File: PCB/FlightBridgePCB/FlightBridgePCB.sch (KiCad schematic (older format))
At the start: 11 parts, among them J1 Raspberry_Pi_2_3, J2 AVR-ISP-6, U1 ATmega128A-AU, Y1 Crystal

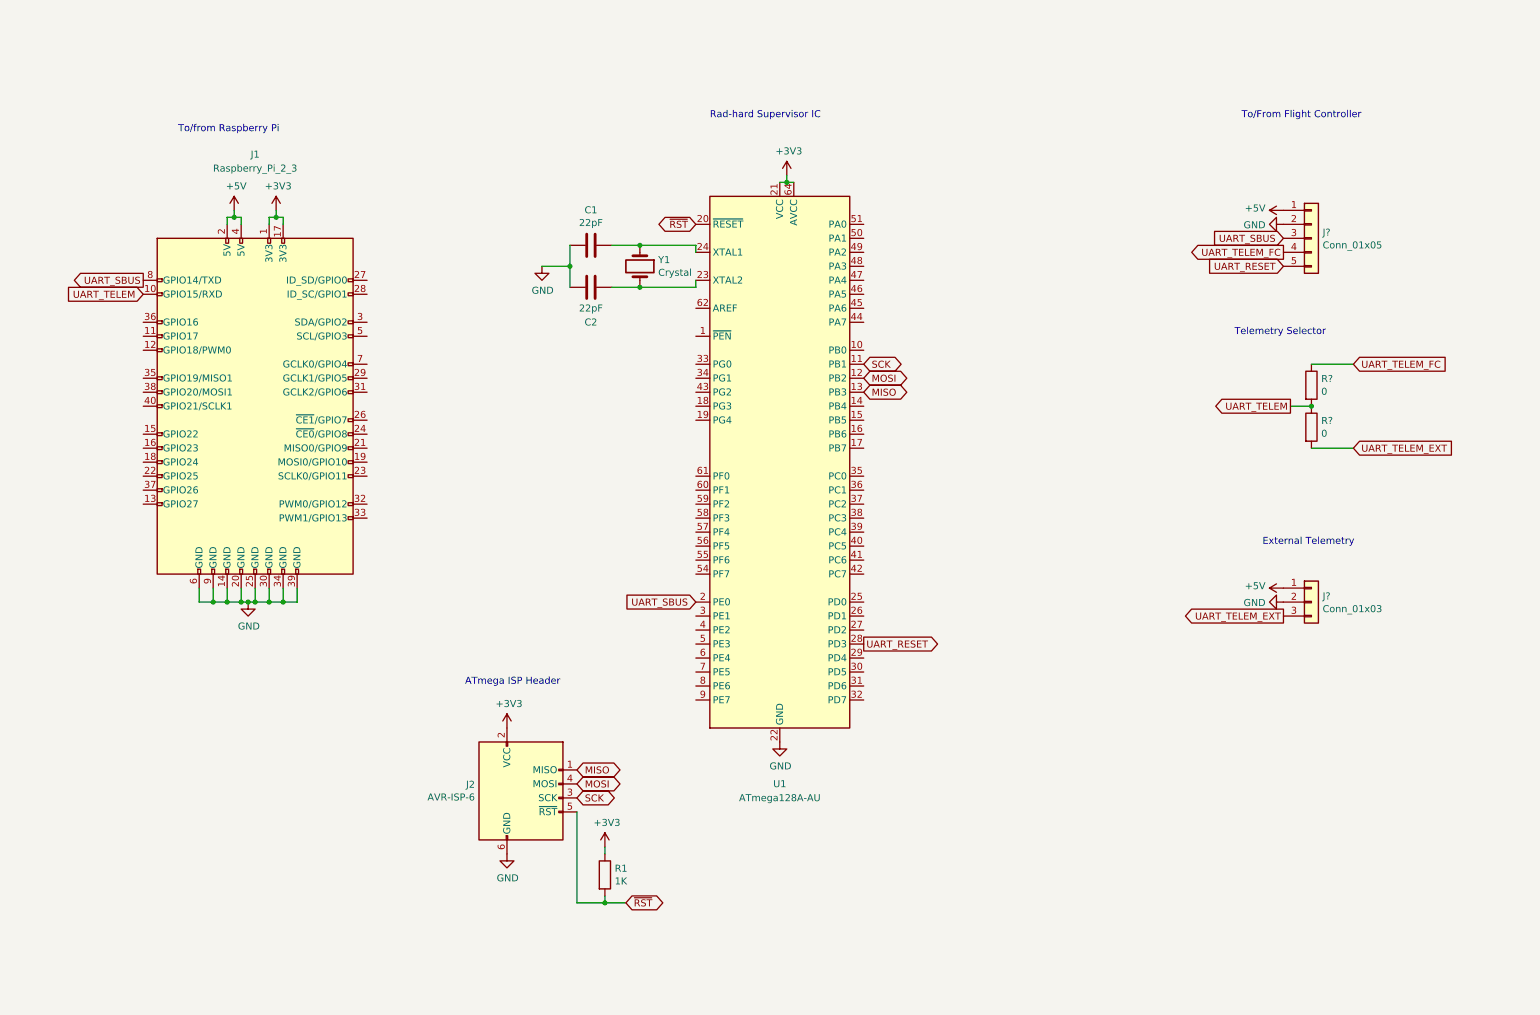
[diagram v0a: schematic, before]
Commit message: First Full PCB
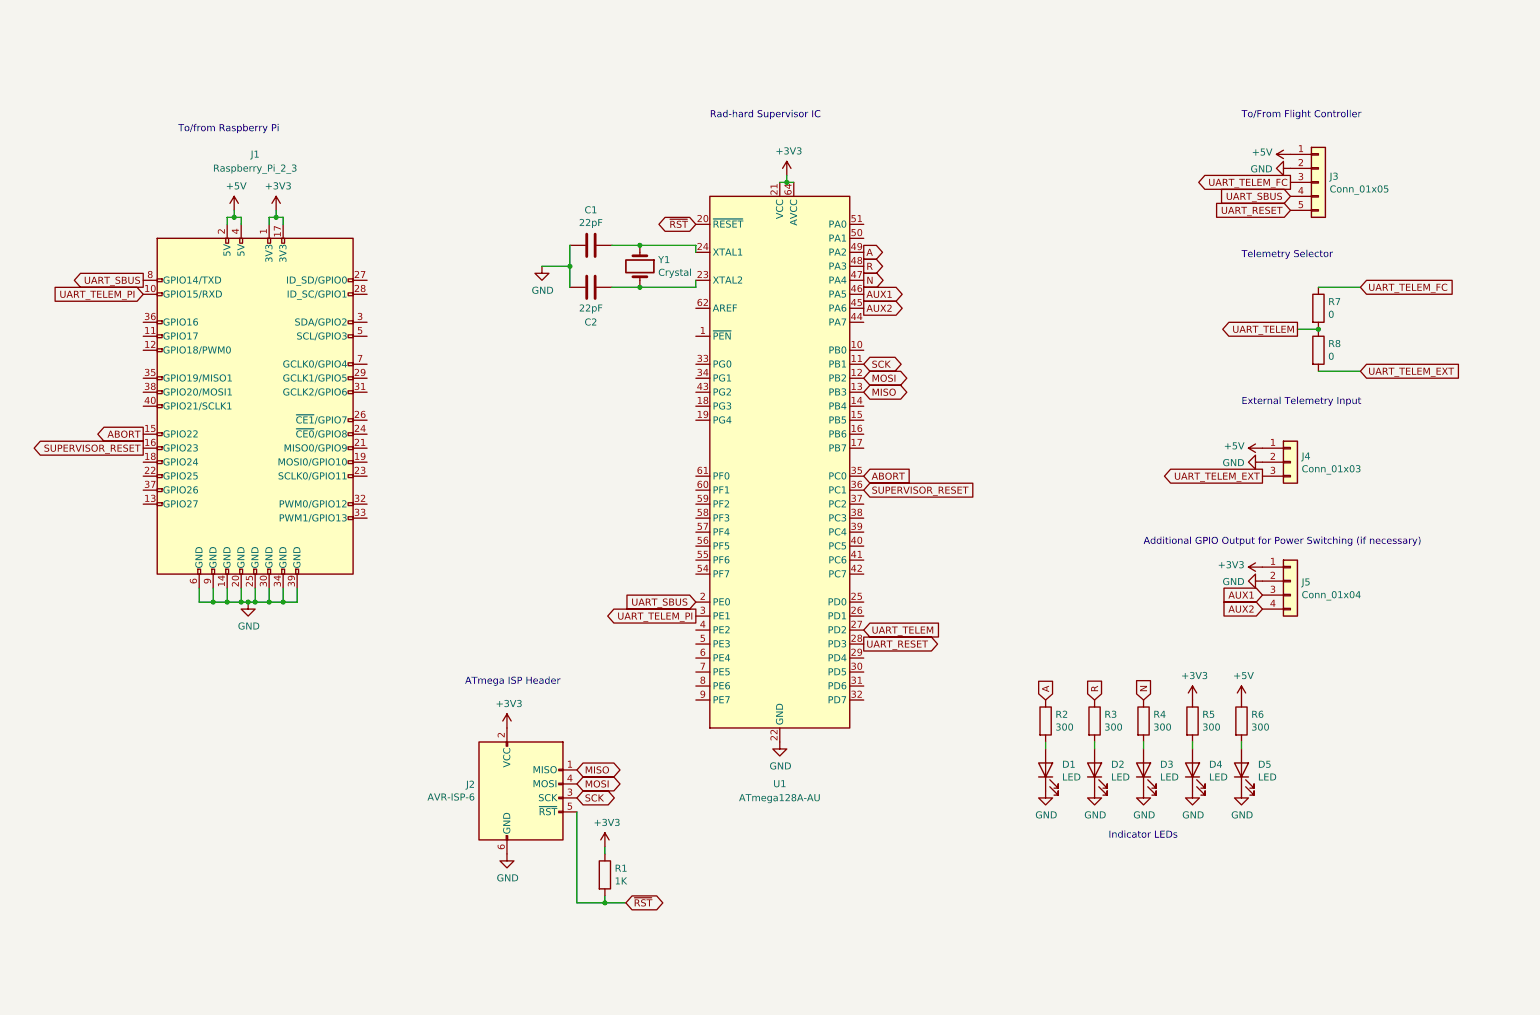
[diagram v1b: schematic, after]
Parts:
- added D1, D2, D3, D4, D5: LED, LED_SMD:LED_0805_2012Metric_Castellated, symbol Device:LED
- added J5: Conn_01x04, Connector_PinHeader_2.54mm:PinHeader_1x04_P2.54mm_Horizontal, symbol Connector_Generic:Conn_01x04
- added R2, R3, R4, R5, R6: 300, Resistor_SMD:R_0805_2012Metric_Pad1.20x1.40mm_HandSolder, symbol Device:R
- J3: renamed from J?; footprint (none) -> Connector_PinHeader_2.54mm:PinHeader_1x05_P2.54mm_Horizontal
- J4: renamed from J?; footprint (none) -> Connector_PinHeader_2.54mm:PinHeader_1x03_P2.54mm_Horizontal
- R7, R8: renamed from R?; footprint (none) -> Resistor_SMD:R_0805_2012Metric_Pad1.20x1.40mm_HandSolder
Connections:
- net +3V3: now also J5.1 (Pin_1), R5.1
- net +5V: now also R6.1
- net GND: now also D1.1 (K), D2.1 (K), D3.1 (K), D4.1 (K), D5.1 (K), J5.2 (Pin_2)
- net UART_SBUS: now also J3.4 (Pin_4); no longer J3.3 (Pin_3)
- net UART_TELEM: now also U1.27 (PD2); no longer J1.10 (GPIO15/RXD)
- net UART_TELEM_FC: now also J3.3 (Pin_3); no longer J3.4 (Pin_4)
- net UART_TELEM_PI: now reaches U1.3 (PE1)
- net UART_TELEM_PI: now also J1.10 (GPIO15/RXD)
- net ABORT: now reaches U1.35 (PC0)
- net ABORT: now also J1.15 (GPIO22)
- net SUPERVISOR_RESET: now reaches U1.36 (PC1)
- net SUPERVISOR_RESET: now also J1.16 (GPIO23)
- net AUX2: now reaches U1.45 (PA6)
- net AUX2: now also J5.4 (Pin_4)
- net AUX1: now reaches U1.46 (PA5)
- net AUX1: now also J5.3 (Pin_3)
- net N: now reaches U1.47 (PA4)
- net N: now also R4.1
- net R: now reaches U1.48 (PA3)
- net R: now also R3.1
- net A: now reaches U1.49 (PA2)
- net A: now also R2.1
- new net: D3.2 (A), R4.2
- new net: D4.2 (A), R5.2
- new net: D5.2 (A), R6.2
- new net: D2.2 (A), R3.2
- new net: D1.2 (A), R2.2
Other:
- note added: "Additional GPIO Output for Power Switching (if necessary)\n"
- note added: "External Telemetry Input\n"
- note added: "Indicator LEDs\n"
- note removed: "External Telemetry"
- moved on the sheet: J3, J4, R7, R8

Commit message: First PCB to be Built
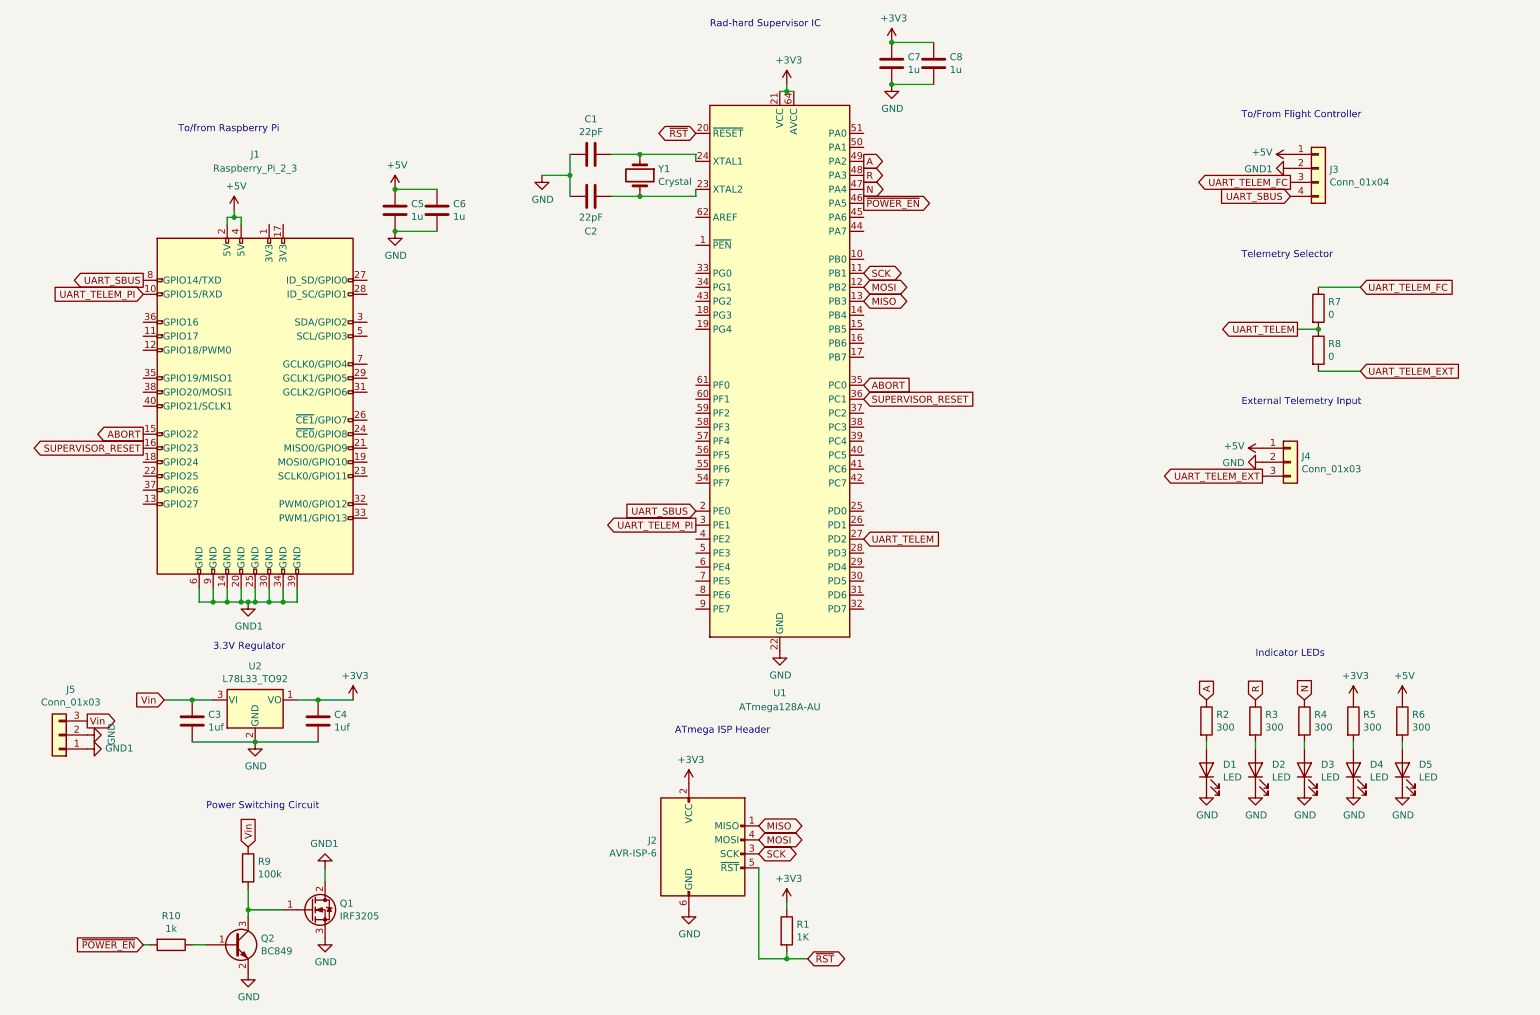
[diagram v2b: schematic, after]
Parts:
- removed J3: Conn_01x05, Connector_PinHeader_2.54mm:PinHeader_1x05_P2.54mm_Horizontal, symbol Connector_Generic:Conn_01x05
- removed J5: Conn_01x04, Connector_PinHeader_2.54mm:PinHeader_1x04_P2.54mm_Horizontal, symbol Connector_Generic:Conn_01x04
- added C3, C4: 1uf, Capacitor_SMD:C_0805_2012Metric_Pad1.18x1.45mm_HandSolder, symbol Device:C
- added C5, C6, C7, C8: 1u, Capacitor_SMD:C_0805_2012Metric_Pad1.18x1.45mm_HandSolder, symbol Device:C
- added J3: Conn_01x04, Connector_PinHeader_2.54mm:PinHeader_1x04_P2.54mm_Horizontal, symbol Connector_Generic:Conn_01x04
- added J5: Conn_01x03, FlightBridgePCB:ELECTRICAL_Connection, symbol Connector_Generic:Conn_01x03
- added Q1: IRF3205, Package_TO_SOT_THT:TO-220-3_Vertical, symbol Transistor_FET:IRF3205
- added Q2: BC849, Package_TO_SOT_SMD:SOT-23, symbol Transistor_BJT:BC849
- added R10: 1k, Resistor_SMD:R_0805_2012Metric_Pad1.20x1.40mm_HandSolder, symbol Device:R
- added R9: 100k, Resistor_SMD:R_0805_2012Metric_Pad1.20x1.40mm_HandSolder, symbol Device:R
- added U2: L78L33_TO92, Package_TO_SOT_THT:TO-92_Inline, symbol Regulator_Linear:L78L33_TO92
- J4: footprint Connector_PinHeader_2.54mm:PinHeader_1x03_P2.54mm_Horizontal -> FlightBridgePCB:EXTERNAL_TELEM
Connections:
- net +3V3: now also C4.1, C7.1, C8.1, U2.1 (VO); no longer J1.1 (3V3), J1.17 (3V3)
- net +5V: now also C5.1, C6.1, J3.1 (Pin_1)
- net GND: now also C3.2, C4.2, C5.2, C6.2, C7.2, C8.2, J5.2 (Pin_2), Q1.3 (S), Q2.2 (E), U2.2 (GND); no longer J1.14 (GND), J1.20 (GND), J1.25 (GND), J1.30 (GND), J1.34 (GND), J1.39 (GND), J1.6 (GND), J1.9 (GND)
- net UART_SBUS: now also J3.4 (Pin_4)
- net UART_TELEM_FC: now also J3.3 (Pin_3)
- net AUX1 renamed ~POWER_EN~
- net ~POWER_EN~: now also R10.2
- net AUX2: no longer names the net of U1.45 (PA6)
- net UART_RESET: no longer names the net of U1.28 (PD3)
- new net: Q1.1 (G), Q2.3 (C), R9.2
- new net: Q2.1 (B), R10.1
- new net GND1: J1.14 (GND), J1.20 (GND), J1.25 (GND), J1.30 (GND), J1.34 (GND), J1.39 (GND), J1.6 (GND), J1.9 (GND), J3.2 (Pin_2), J5.1 (Pin_1), Q1.2 (D)
- new net Vin: C3.1, J5.3 (Pin_3), R9.1, U2.3 (VI)
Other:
- note added: "3.3V Regulator\n"
- note added: "Power Switching Circuit\n\n\n"
- note removed: "Additional GPIO Output for Power Switching (if necessary)\n"
- moved on the sheet: C1, C2, D1, D2, D3, D4, D5, J2, R1, R2, R3, R4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
